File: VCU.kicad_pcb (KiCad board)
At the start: 2 copper layers, 44.3 x 40.3 mm, 36 parts, among them J2 2x3_Conn, J3 USB_C_Receptacle_USB2.0_14P, U1 ESP32-S3-WROOM-1, U2 LM1117DT-3.3, U3 SN65HVD230, U4 USBLC6-2SC6, U6 MCP6001-OT

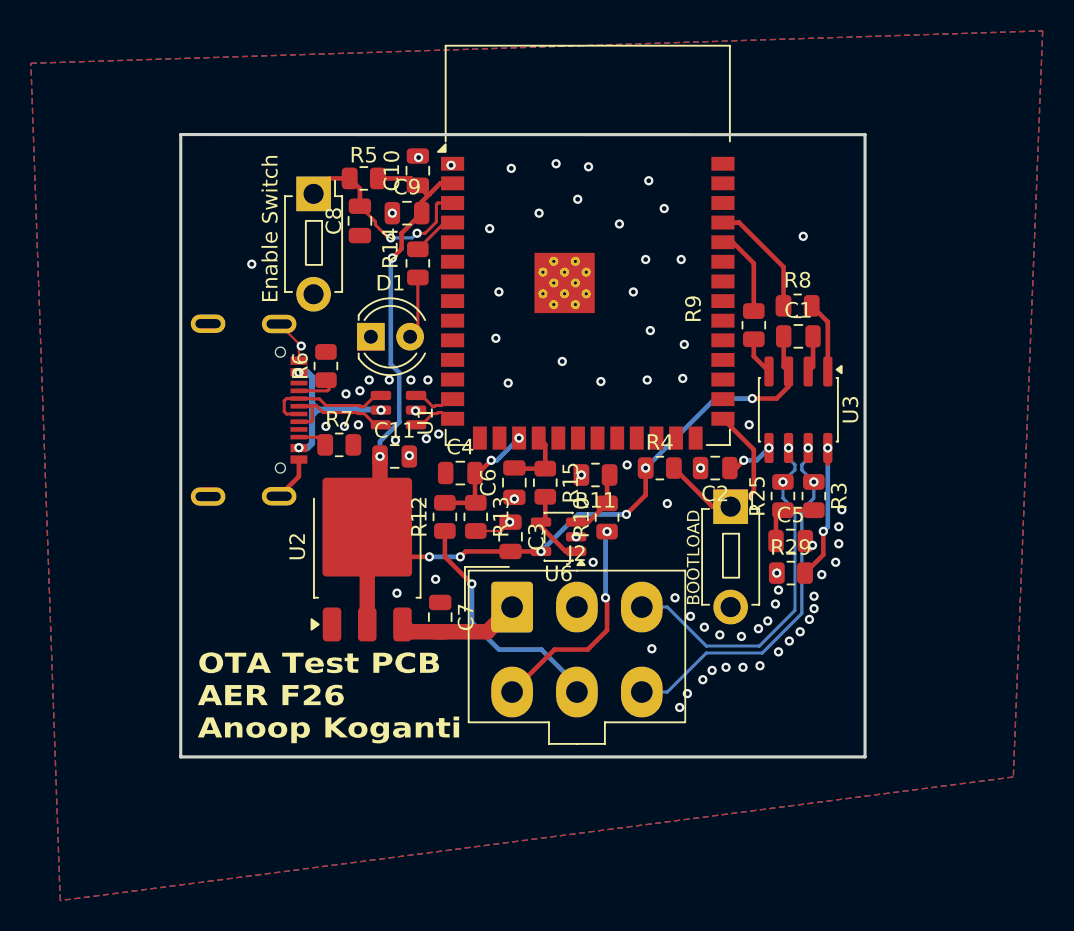
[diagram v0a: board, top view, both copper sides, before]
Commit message: Do Layout
Yuh
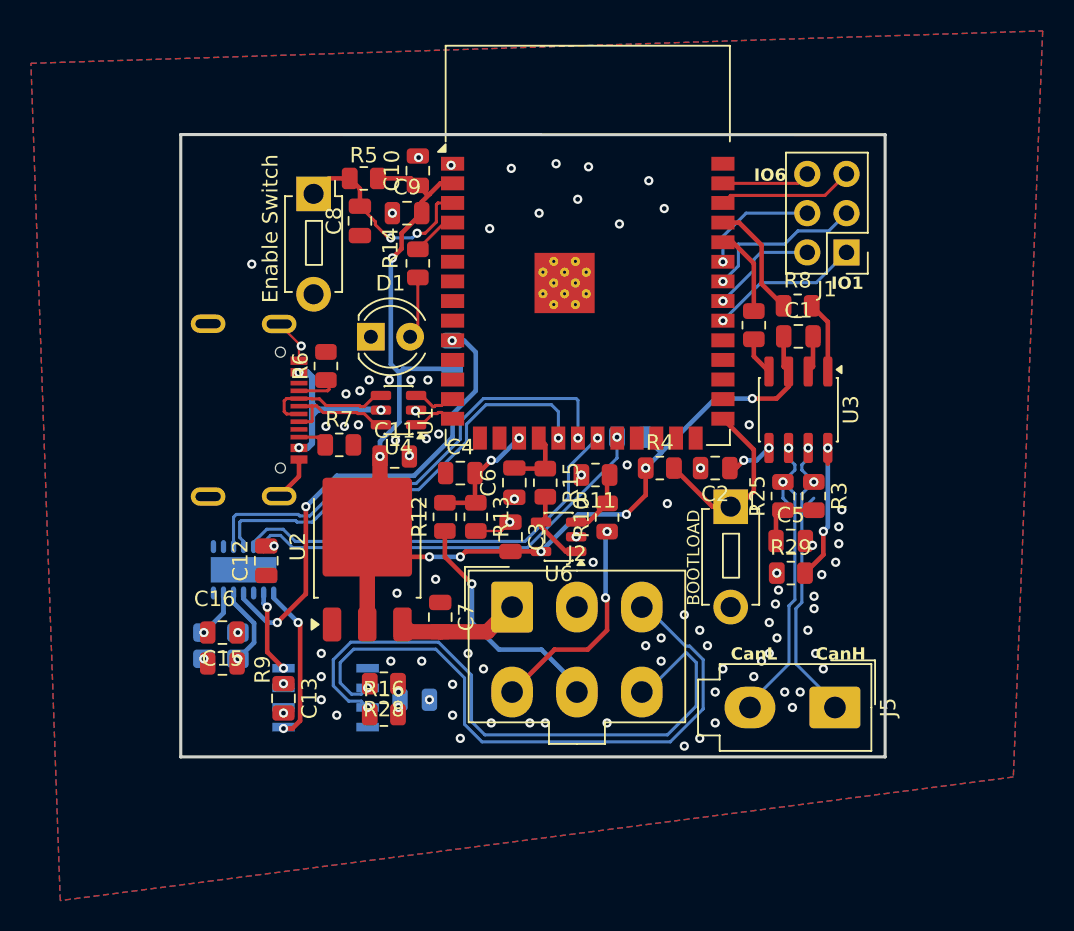
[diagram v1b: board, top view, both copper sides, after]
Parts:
- added C12: 100 nF, Capacitor_SMD:C_0805_2012Metric, F.Cu at (72.4, 69.5)
- added C13: 100 nF, Capacitor_SMD:C_0805_2012Metric, F.Cu at (73.6, 78.4)
- added C14: 100 nF, Capacitor_SMD:C_0805_2012Metric, B.Cu at (82.0, 78.5)
- added C15: 27pF, Capacitor_SMD:C_0805_2012Metric, F.Cu at (69.6, 74.2)
- added C16: 27pF, Capacitor_SMD:C_0805_2012Metric, F.Cu at (69.6, 76.2)
- added J1: Conn_02x03_Top_Bottom, Connector_PinHeader_2.54mm:PinHeader_2x03_P2.54mm_Vertical, F.Cu at (110.0, 49.5)
- added J5: Conn_01x02, Connector_Molex:Molex_Mini-Fit_Jr_5566-02A_2x01_P4.20mm_Vertical, F.Cu at (109.2, 79.0)
- added R16: 60, Resistor_SMD:R_0805_2012Metric, F.Cu at (80.1, 79.5)
- added R26: 10k, Resistor_SMD:R_0805_2012Metric, B.Cu at (96.1, 61.5)
- added R27: 10k, Resistor_SMD:R_0805_2012Metric, B.Cu at (84.5, 56.2)
- added R28: 60, Resistor_SMD:R_0805_2012Metric, F.Cu at (80.1, 77.5)
- added U5: MCP2518FD-xQBB, Package_DFN_QFN:DFN-14-1EP_3x4.5mm_P0.65mm_EP1.65x4.25mm, B.Cu at (71.0, 70.1)
- added U7: PTCAN3413DR, KiCADv6:SOIC8_D_TEX, B.Cu at (76.3, 78.4)
- added Y1: 40Mhz Crystal, Crystal:Crystal_SMD_3225-4Pin_3.2x2.5mm, B.Cu at (69.5, 75.0)
- U4: footprint SK's_Components:ESD_SOT-23-6 -> Package_TO_SOT_SMD:SOT-23-6
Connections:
- net Vin(12V) renamed Vin(5V)
- C1 pad 2: Net-(U3-GND) -> GND
- C2 pad 1: Net-(U3-Vref) -> +3.3V
- J2 pad 3: CAN- -> /CANFD-
- J2 pad 6: CAN+ -> /CANFD+
- J3 pad S1: GND -> (no net)
- R15 pad 1: GPIO_TEST1 -> Net-(U6--)
- R15 pad 2: Net-(U6--) -> GPIO_TEST1
- U1 pad 10: unconnected-(U1-IO17-Pad10) -> /INT
- U1 pad 19: unconnected-(U1-IO11-Pad19) -> /MOSI
- U1 pad 20: unconnected-(U1-IO12-Pad20) -> /SPIClk
- U1 pad 21: unconnected-(U1-IO13-Pad21) -> /MISO
- U1 pad 22: unconnected-(U1-IO14-Pad22) -> /CS
- U1 pad 32: unconnected-(U1-IO39-Pad32) -> /IO1
- U1 pad 33: unconnected-(U1-IO40-Pad33) -> /IO2
- U1 pad 34: unconnected-(U1-IO41-Pad34) -> /IO3
- U1 pad 35: unconnected-(U1-IO42-Pad35) -> /IO4
- U1 pad 38: unconnected-(U1-IO2-Pad38) -> /IO5
- U1 pad 39: unconnected-(U1-IO1-Pad39) -> /IO6
- U3 pad 2: Net-(U3-GND) -> GND
- U3 pad 5: Net-(U3-Vref) -> +3.3V
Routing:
- net /CANFD+: track 0.00 -> 41.1 mm, vias 0 -> 1
- net /CANFD-: track 0.00 -> 41.1 mm, vias 0 -> 1
- net /INT: track 0.00 -> 30.8 mm, vias 0 -> 3
- net /SPIClk: track 0.00 -> 30.6 mm, vias 0 -> 1
- net /MOSI: track 0.00 -> 28.1 mm, vias 0 -> 1
- net /CS: track 0.00 -> 27.4 mm, vias 0 -> 1
- net /MISO: track 0.00 -> 27.2 mm, vias 0 -> 1
- net /IO3: track 0.00 -> 10.7 mm, vias 0 -> 1
- net /TX: track 0.00 -> 10.3 mm, vias 0 -> 2
- net /IO1: track 0.00 -> 9.83 mm, vias 0 -> 1
- net /IO5: track 0.00 -> 8.78 mm
- net +3.3V: track 72.6 -> 80.7 mm, vias 8 -> 12
- net /IO4: track 0.00 -> 7.73 mm, vias 0 -> 1
- net /IO2: track 0.00 -> 7.17 mm, vias 0 -> 1
- net /IO6: track 0.00 -> 5.71 mm
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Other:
- board size 44.3 x 40.3 mm -> 45.6 x 40.3 mm
- board text added: "CanH"
- board text added: "CanL"
- board text added: "GND"
- board text added: "GPIO1"
- board text added: "GPIO2"
- board text added: "IO1"
- board text added: "IO6"
- board text added: "Vin"
